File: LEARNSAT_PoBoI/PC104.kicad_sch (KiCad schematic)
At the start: 28 parts, among them J1 FTSH-105-01-L-DV-K-P-TR, P1 22-28-4036, SW3 TS04-66-43-BK-100-SMT

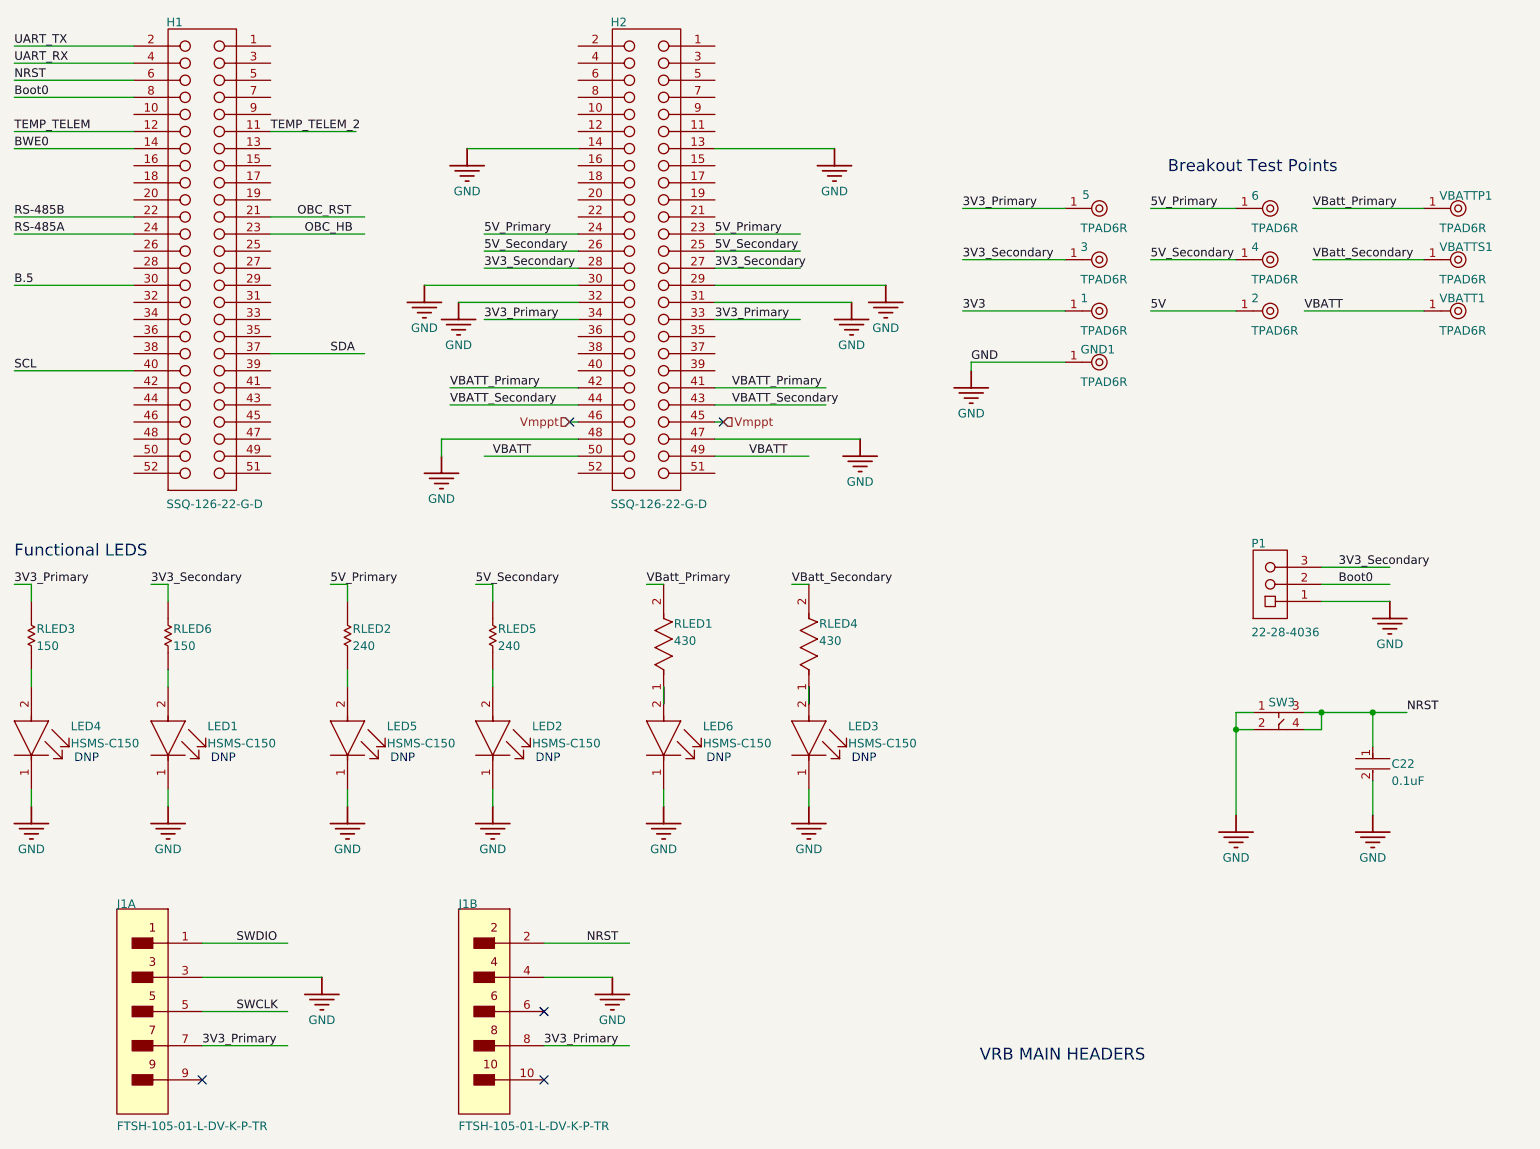
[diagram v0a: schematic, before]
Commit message: Added footprints
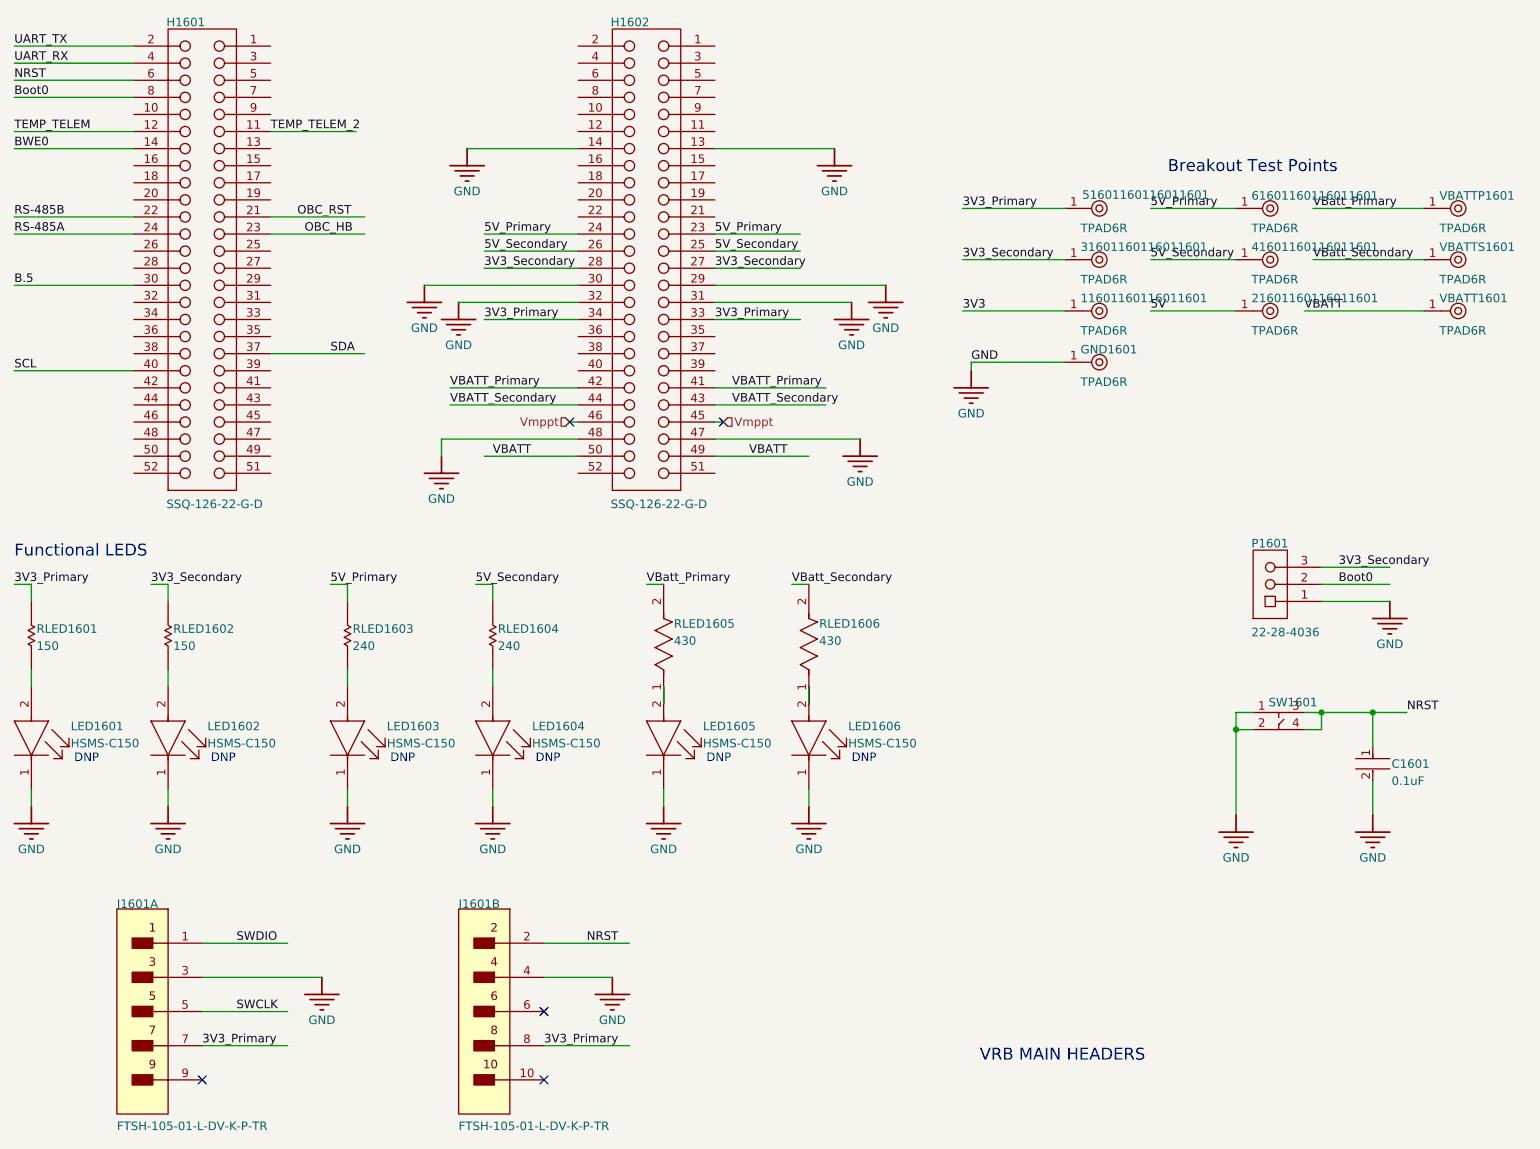
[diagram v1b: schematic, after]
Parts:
- 11601160116011601: renamed from 1; footprint TP06R -> TestPoint:TestPoint_Pad_D1.0mm
- 21601160116011601: renamed from 2; footprint TP06R -> TestPoint:TestPoint_Pad_D1.0mm
- 31601160116011601: renamed from 3; footprint TP06R -> TestPoint:TestPoint_Pad_D1.0mm
- 41601160116011601: renamed from 4; footprint TP06R -> TestPoint:TestPoint_Pad_D1.0mm
- 51601160116011601: renamed from 5; footprint TP06R -> TestPoint:TestPoint_Pad_D1.0mm
- 61601160116011601: renamed from 6; footprint TP06R -> TestPoint:TestPoint_Pad_D1.0mm
- C1601: renamed from C22; footprint FP-C0603-CJ-MFG -> Capacitor_SMD:C_0603_1608Metric
- GND1601: renamed from GND1; footprint TP06R -> TestPoint:TestPoint_Pad_D1.0mm
- H1601: renamed from H1; footprint SMTC-SSQ-126-22-X-D -> SSQ-126-X-G-D:SAMTEC_SSQ-126-X-G-D
- H1602: renamed from H2; footprint SMTC-SSQ-126-22-X-D -> SSQ-126-X-G-D:SAMTEC_SSQ-126-X-G-D
- J1601: renamed from J1; footprint FP-FTSH-105-01-L-DV-K-P-T-MFG -> FTSH-105-01-X-DV-K-P-X:SAMTEC_FTSH-105-01-X-DV-K-P-X
- LED1601: renamed from LED4; footprint FP-HSMS-C150-MFG -> LED_APTL3216CGCK:LED_APTL3216CGCK
- LED1602: renamed from LED1; footprint FP-HSMS-C150-MFG -> LED_APTL3216CGCK:LED_APTL3216CGCK
- LED1603: renamed from LED5; footprint FP-HSMS-C150-MFG -> LED_APTL3216CGCK:LED_APTL3216CGCK
- LED1604: renamed from LED2; footprint FP-HSMS-C150-MFG -> LED_APTL3216CGCK:LED_APTL3216CGCK
- LED1605: renamed from LED6; footprint FP-HSMS-C150-MFG -> LED_APTL3216CGCK:LED_APTL3216CGCK
- LED1606: renamed from LED3; footprint FP-HSMS-C150-MFG -> LED_APTL3216CGCK:LED_APTL3216CGCK
- P1601: renamed from P1; footprint 22-28-4036-Footprint-1 -> SSQ-126-X-G-D:SAMTEC_SSQ-126-X-G-D
- RLED1601: renamed from RLED3; footprint RESC1608X55X25ML10T15 -> Resistor_SMD:R_0603_1608Metric
- RLED1602: renamed from RLED6; footprint RESC1608X55X25ML10T15 -> Resistor_SMD:R_0603_1608Metric
- RLED1603: renamed from RLED2; footprint RESC1608X55X30NL20T20 -> Resistor_SMD:R_0603_1608Metric
- RLED1604: renamed from RLED5; footprint RESC1608X55X30NL20T20 -> Resistor_SMD:R_0603_1608Metric
- RLED1605: renamed from RLED1; footprint FP-CRCW0603-e3-IPC_B -> Resistor_SMD:R_0603_1608Metric
- RLED1606: renamed from RLED4; footprint FP-CRCW0603-e3-IPC_B -> Resistor_SMD:R_0603_1608Metric
- SW1601: renamed from SW3; footprint SOP127P600-8N -> TS04-66-43-BK-100-SMT:SW_TS04-66-43-BK-100-SMT
- VBATT1601: renamed from VBATT1; footprint TP06R -> TestPoint:TestPoint_Pad_D1.0mm
- VBATTP1601: renamed from VBATTP1; footprint TP06R -> TestPoint:TestPoint_Pad_D1.0mm
- VBATTS1601: renamed from VBATTS1; footprint TP06R -> TestPoint:TestPoint_Pad_D1.0mm

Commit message: Add files via upload
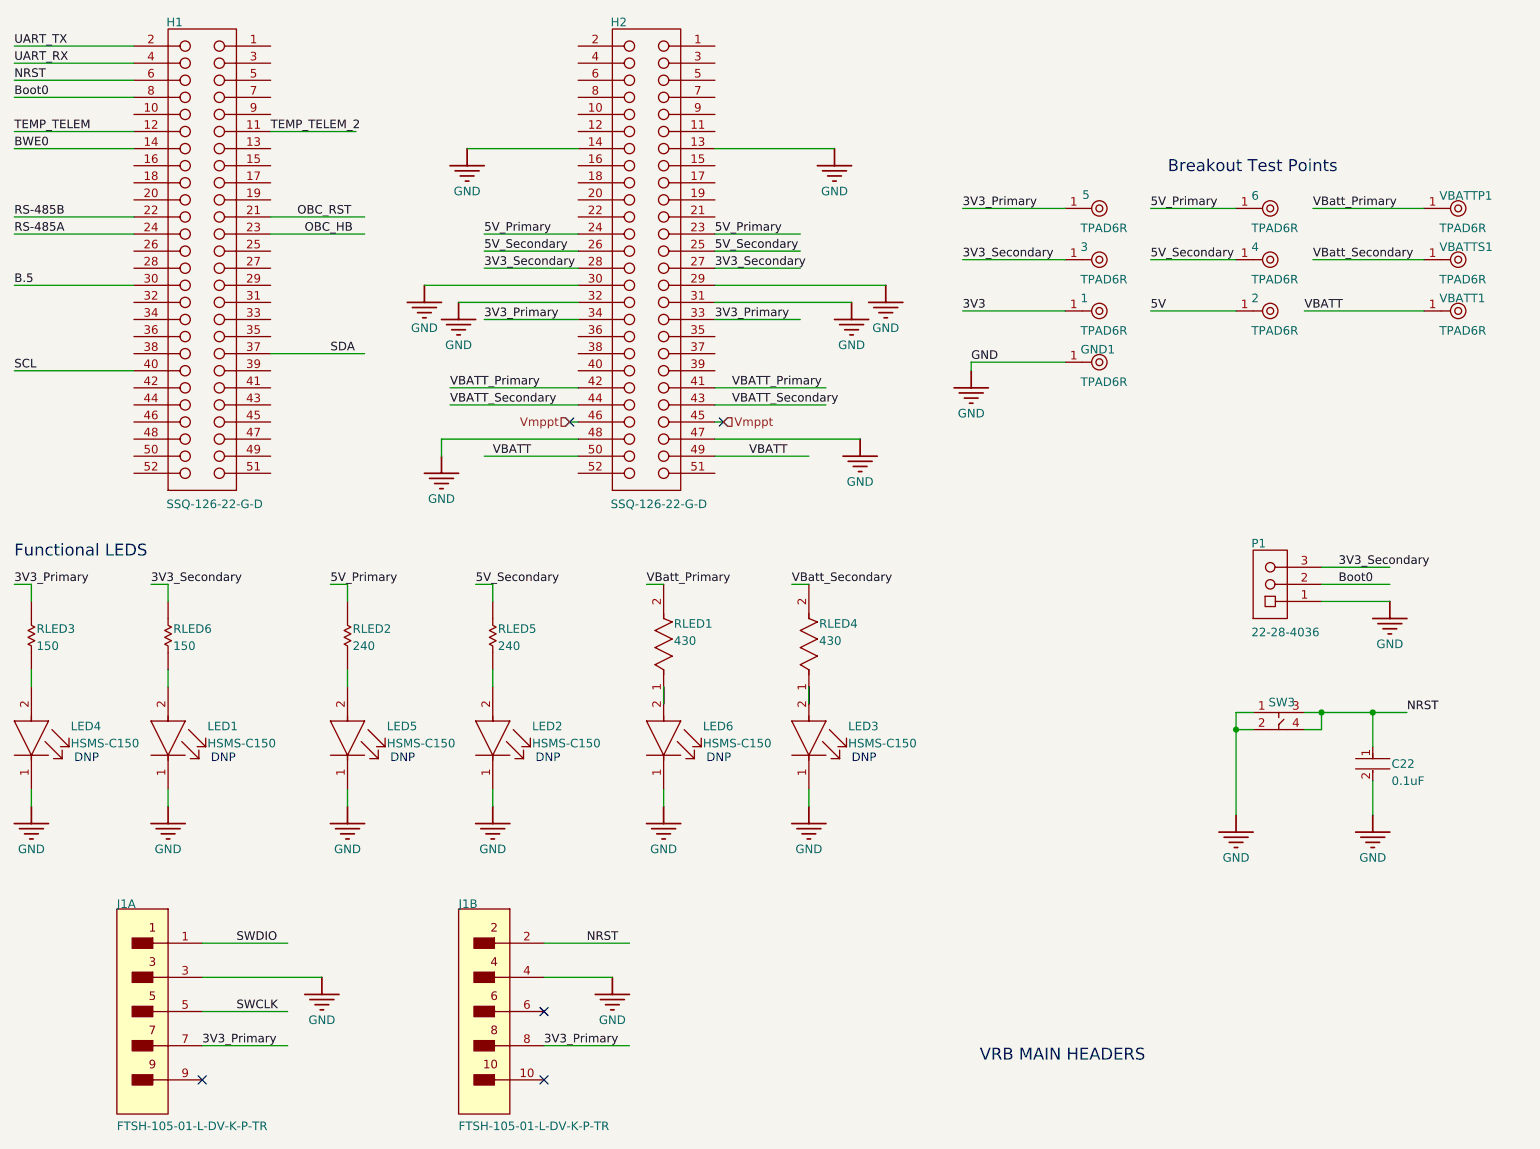
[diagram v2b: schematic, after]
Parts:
- 1: renamed from 11601160116011601; footprint TestPoint:TestPoint_Pad_D1.0mm -> TP06R
- 2: renamed from 21601160116011601; footprint TestPoint:TestPoint_Pad_D1.0mm -> TP06R
- 3: renamed from 31601160116011601; footprint TestPoint:TestPoint_Pad_D1.0mm -> TP06R
- 4: renamed from 41601160116011601; footprint TestPoint:TestPoint_Pad_D1.0mm -> TP06R
- 5: renamed from 51601160116011601; footprint TestPoint:TestPoint_Pad_D1.0mm -> TP06R
- 6: renamed from 61601160116011601; footprint TestPoint:TestPoint_Pad_D1.0mm -> TP06R
- C22: renamed from C1601; footprint Capacitor_SMD:C_0603_1608Metric -> FP-C0603-CJ-MFG
- GND1: renamed from GND1601; footprint TestPoint:TestPoint_Pad_D1.0mm -> TP06R
- H1: renamed from H1601; footprint SSQ-126-X-G-D:SAMTEC_SSQ-126-X-G-D -> SMTC-SSQ-126-22-X-D
- H2: renamed from H1602; footprint SSQ-126-X-G-D:SAMTEC_SSQ-126-X-G-D -> SMTC-SSQ-126-22-X-D
- J1: renamed from J1601; footprint FTSH-105-01-X-DV-K-P-X:SAMTEC_FTSH-105-01-X-DV-K-P-X -> FP-FTSH-105-01-L-DV-K-P-T-MFG
- LED1: renamed from LED1602; footprint LED_APTL3216CGCK:LED_APTL3216CGCK -> FP-HSMS-C150-MFG
- LED2: renamed from LED1604; footprint LED_APTL3216CGCK:LED_APTL3216CGCK -> FP-HSMS-C150-MFG
- LED3: renamed from LED1606; footprint LED_APTL3216CGCK:LED_APTL3216CGCK -> FP-HSMS-C150-MFG
- LED4: renamed from LED1601; footprint LED_APTL3216CGCK:LED_APTL3216CGCK -> FP-HSMS-C150-MFG
- LED5: renamed from LED1603; footprint LED_APTL3216CGCK:LED_APTL3216CGCK -> FP-HSMS-C150-MFG
- LED6: renamed from LED1605; footprint LED_APTL3216CGCK:LED_APTL3216CGCK -> FP-HSMS-C150-MFG
- P1: renamed from P1601; footprint SSQ-126-X-G-D:SAMTEC_SSQ-126-X-G-D -> 22-28-4036-Footprint-1
- RLED1: renamed from RLED1605; footprint Resistor_SMD:R_0603_1608Metric -> FP-CRCW0603-e3-IPC_B
- RLED2: renamed from RLED1603; footprint Resistor_SMD:R_0603_1608Metric -> RESC1608X55X30NL20T20
- RLED3: renamed from RLED1601; footprint Resistor_SMD:R_0603_1608Metric -> RESC1608X55X25ML10T15
- RLED4: renamed from RLED1606; footprint Resistor_SMD:R_0603_1608Metric -> FP-CRCW0603-e3-IPC_B
- RLED5: renamed from RLED1604; footprint Resistor_SMD:R_0603_1608Metric -> RESC1608X55X30NL20T20
- RLED6: renamed from RLED1602; footprint Resistor_SMD:R_0603_1608Metric -> RESC1608X55X25ML10T15
- SW3: renamed from SW1601; footprint TS04-66-43-BK-100-SMT:SW_TS04-66-43-BK-100-SMT -> SOP127P600-8N
- VBATT1: renamed from VBATT1601; footprint TestPoint:TestPoint_Pad_D1.0mm -> TP06R
- VBATTP1: renamed from VBATTP1601; footprint TestPoint:TestPoint_Pad_D1.0mm -> TP06R
- VBATTS1: renamed from VBATTS1601; footprint TestPoint:TestPoint_Pad_D1.0mm -> TP06R
